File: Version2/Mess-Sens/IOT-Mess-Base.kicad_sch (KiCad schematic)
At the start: 25 parts, among them IC1 SHT40I-AD1F-R2, J1 Conn_01x02_Pin, J2 Conn_01x06_Pin, U1 TMP102xxDRL, U10 OPT3001DNPR, U11 HDC2010/DSBGA-6, U12 MMC5633NJL/WLP-4, U13 BH1750FVI-TR, U14 T117W, U15 DS1307Z+, U16 ENS210, U19 MTS4, U3 TLV493D, U4 TMP1075DGK, U5 SHT31-DIS, U6 APDS-9960, U7 QMC6309/WLCSP-4, U9 LTR-303ALS-01

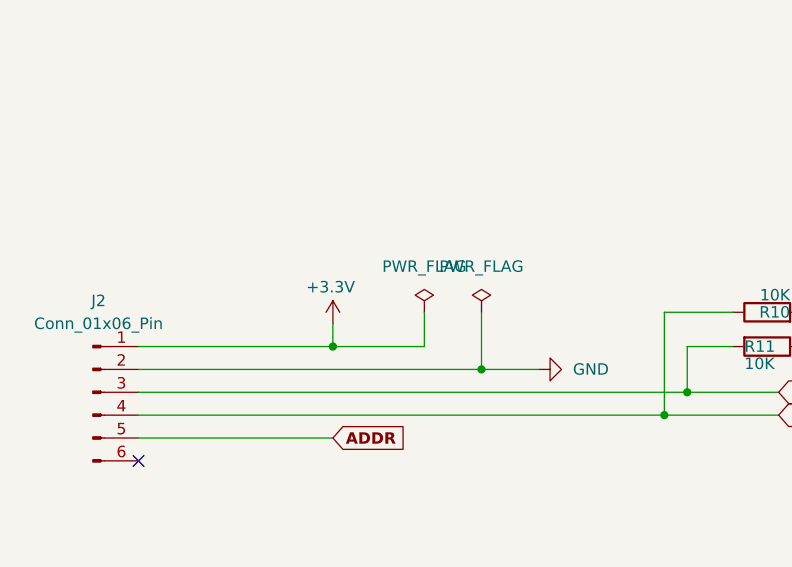
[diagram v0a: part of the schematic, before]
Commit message: update stuff.
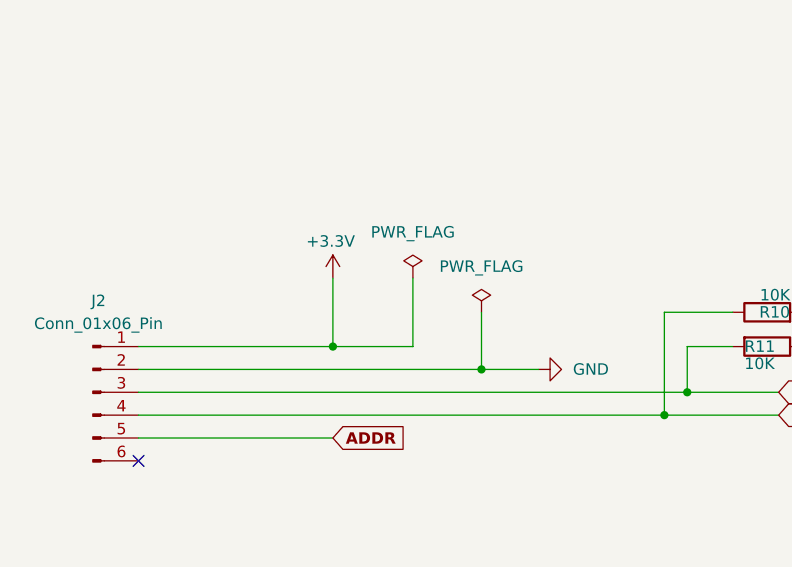
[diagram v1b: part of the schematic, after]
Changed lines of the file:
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@@
 	(wire
 		(pts
-			(xy 80.01 146.05) (xy 80.01 149.86)
+			(xy 78.74 142.24) (xy 78.74 149.86)
 		)
 		(stroke
@@
 	(wire
 		(pts
-			(xy 69.85 149.86) (xy 80.01 149.86)
+			(xy 69.85 149.86) (xy 78.74 149.86)
 		)
 		(stroke
@@
 	(wire
 		(pts
-			(xy 69.85 147.32) (xy 69.85 149.86)
+			(xy 69.85 142.24) (xy 69.85 149.86)
 		)
 		(stroke
@@
 	(symbol
 		(lib_id "power:+3.3V")
-		(at 69.85 147.32 0)
+		(at 69.85 142.24 0)
 		(unit 1)
 		(exclude_from_sim no)
@@
 		(dnp no)
 		(property "Reference" "#PWR015"
-			(at 69.85 151.13 0)
+			(at 69.85 146.05 0)
 			(effects
 				(font
@@
 		)
 		(property "Value" "+3.3V"
-			(at 69.596 143.256 0)
+			(at 69.596 138.176 0)
 			(effects
 				(font
@@
 		)
 		(property "Footprint" ""
-			(at 69.85 147.32 0)
+			(at 69.85 142.24 0)
 			(effects
 				(font
@@
 		)
 		(property "Datasheet" ""
-			(at 69.85 147.32 0)
+			(at 69.85 142.24 0)
 			(effects
 				(font
@@
 		)
 		(property "Description" ""
-			(at 69.85 147.32 0)
+			(at 69.85 142.24 0)
 			(effects
 				(font
@@
 	(symbol
 		(lib_id "power:PWR_FLAG")
-		(at 80.01 146.05 0)
+		(at 78.74 142.24 0)
 		(unit 1)
 		(exclude_from_sim no)
@@
 		(dnp no)
 		(property "Reference" "#FLG02"
-			(at 80.01 144.145 0)
+			(at 78.74 140.335 0)
 			(effects
 				(font
@@
 		)
 		(property "Value" "PWR_FLAG"
-			(at 80.01 140.97 0)
+			(at 78.74 137.16 0)
 			(effects
 				(font
@@
 		)
 		(property "Footprint" ""
-			(at 80.01 146.05 0)
+			(at 78.74 142.24 0)
 			(effects
 				(font
@@
 		)
 		(property "Datasheet" "~"
-			(at 80.01 146.05 0)
+			(at 78.74 142.24 0)
 			(effects
 				(font
@@
 		)
 		(property "Description" "Special symbol for telling ERC where power comes from"
-			(at 80.01 146.05 0)
+			(at 78.74 142.24 0)
 			(effects
 				(font
